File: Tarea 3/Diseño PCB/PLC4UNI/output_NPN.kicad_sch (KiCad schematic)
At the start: 3 parts

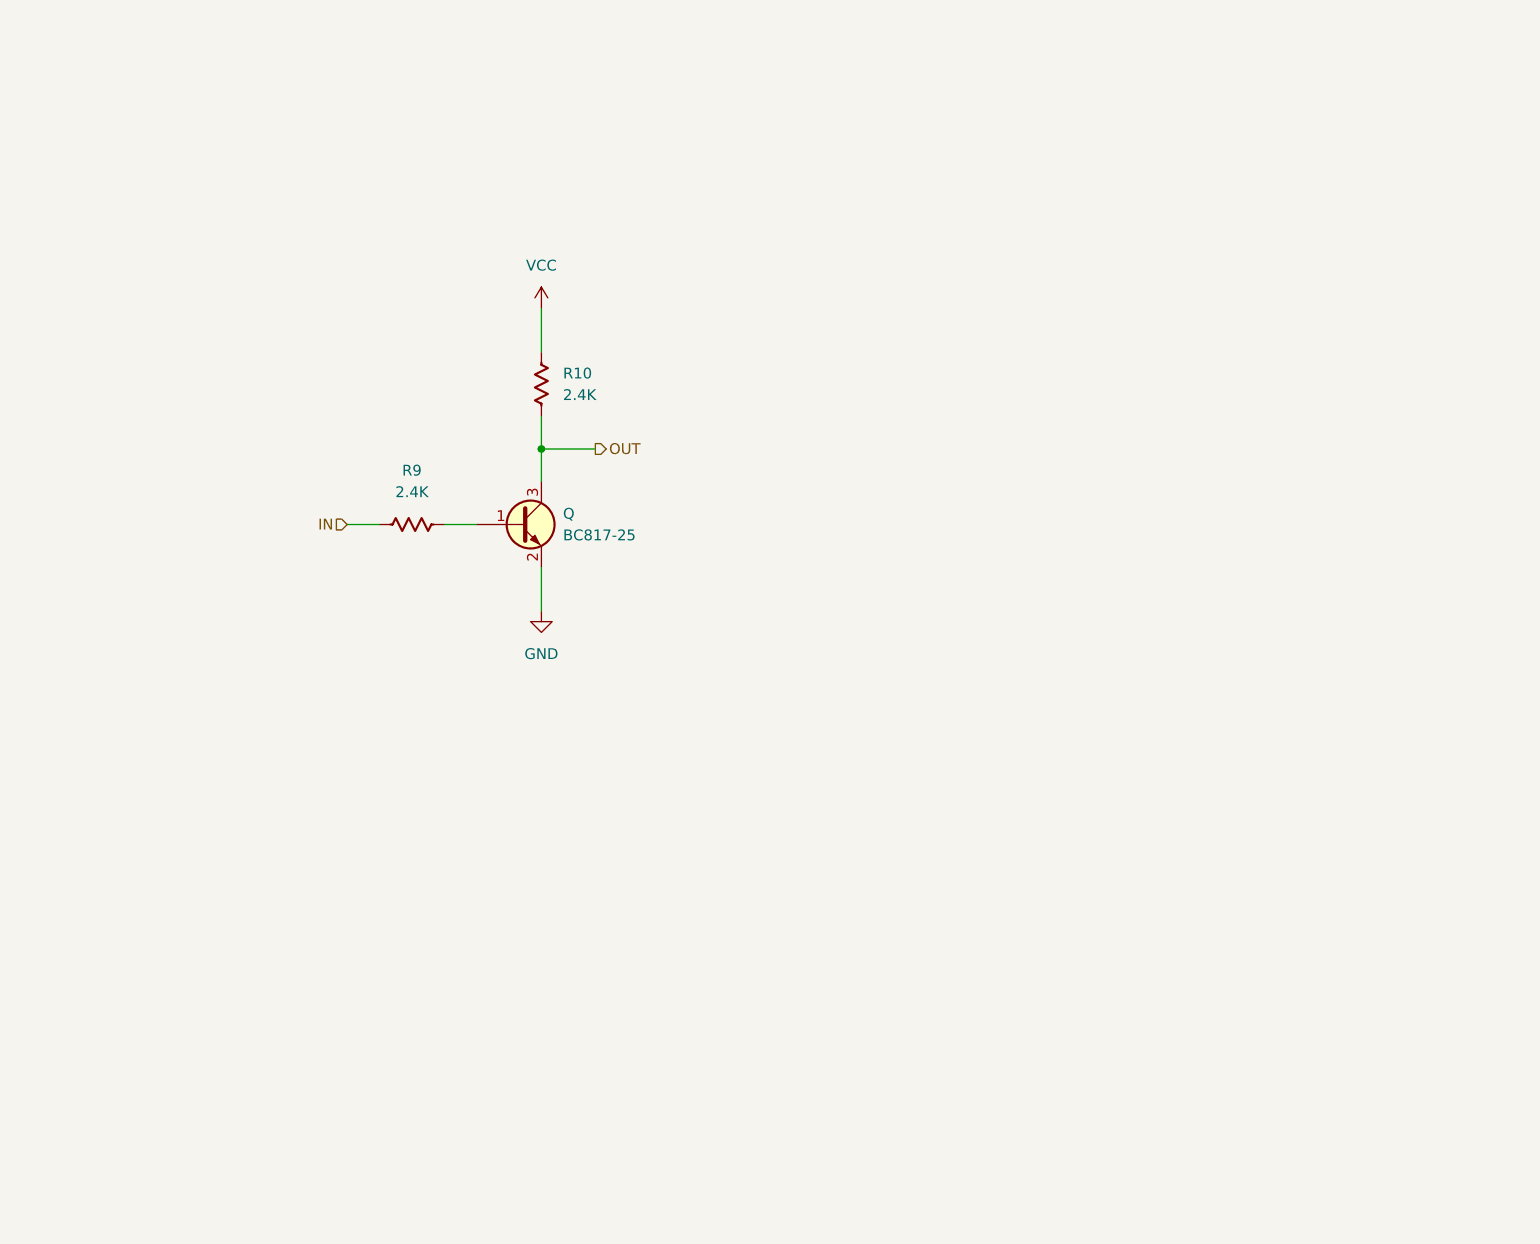
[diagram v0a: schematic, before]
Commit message: Tarea 3
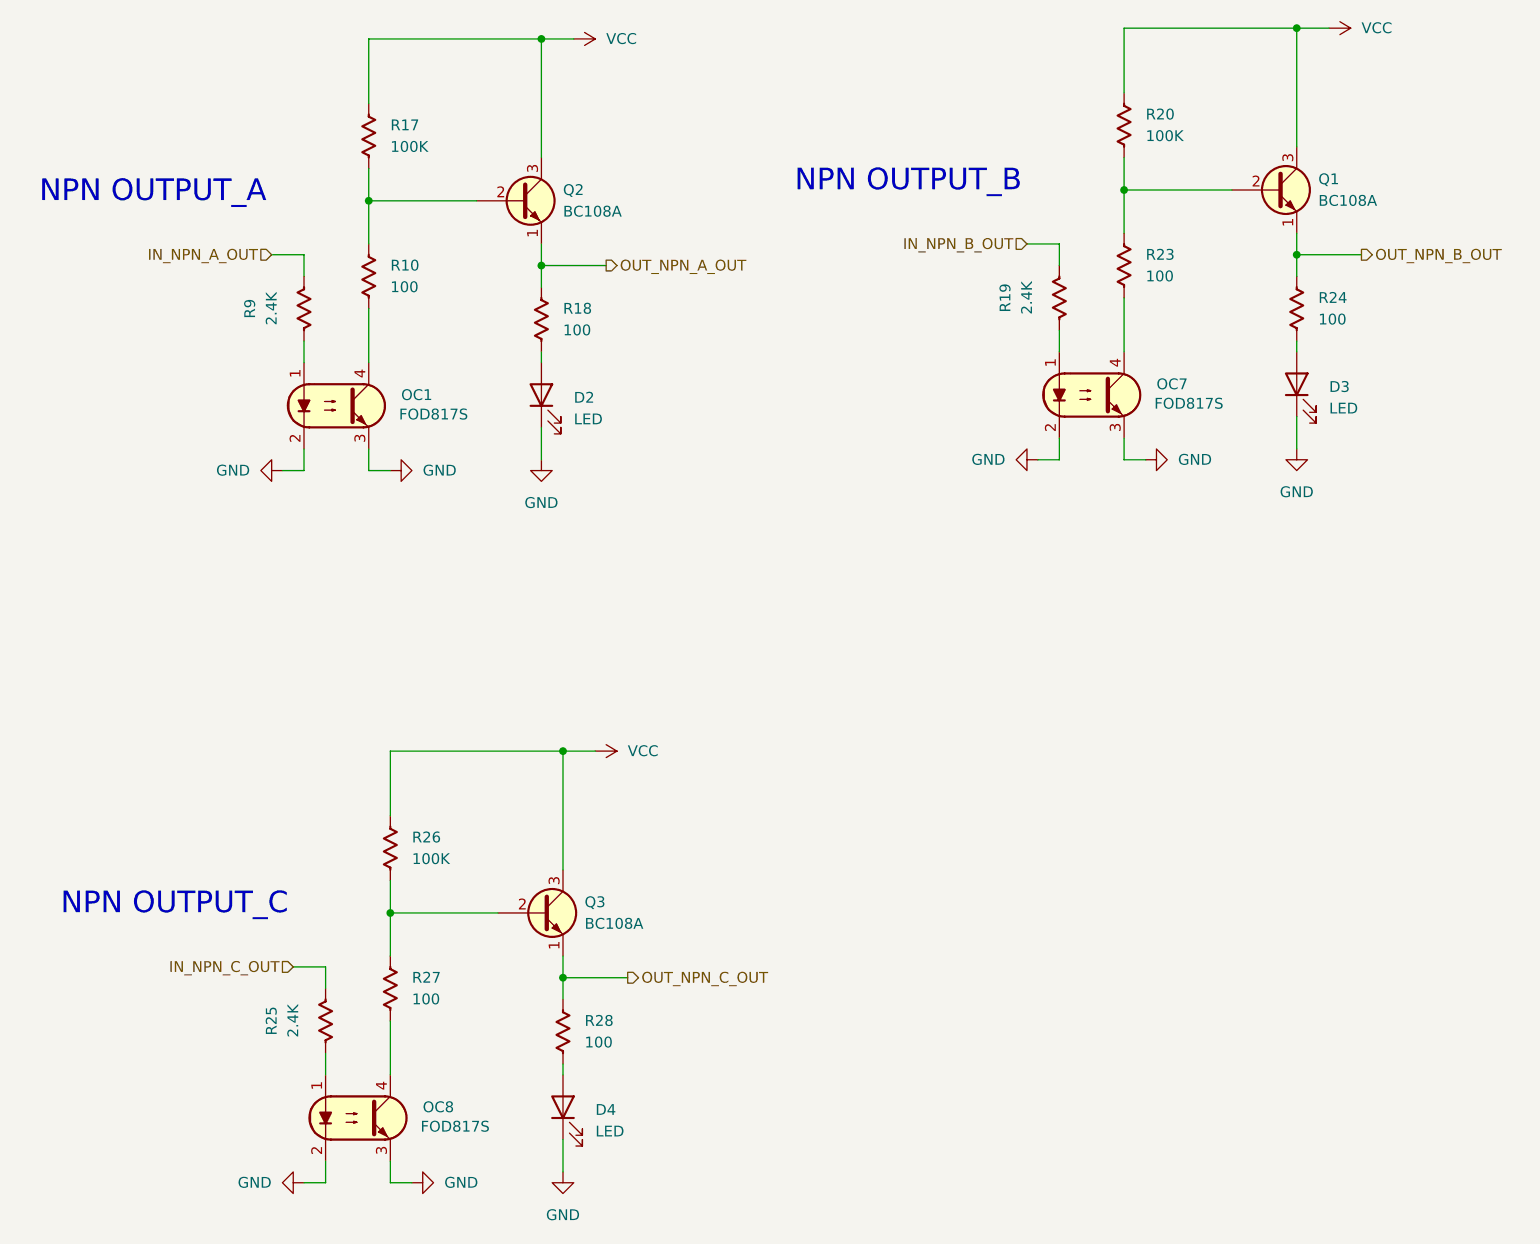
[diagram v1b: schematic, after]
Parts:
- removed Q: BC817-25, PCM_Package_TO_SOT_SMD_AKL:SOT-23, symbol PCM_Transistor_BJT_AKL:BC817-25
- added D2, D3, D4: LED, symbol Device:LED
- added OC1, OC7, OC8: FOD817S, PCM_Package_DIP_AKL:SMDIP-4_W9.53mm, symbol PCM_Optocoupler_AKL:FOD817S
- added Q1, Q2, Q3: BC108A, PCM_Package_TO_SOT_THT_AKL:TO-18-3_EBC, symbol PCM_Transistor_BJT_AKL:BC108A
- added R17, R20, R26: 100K, PCM_Resistor_SMD_AKL:R_0603_1608Metric, symbol PCM_Resistor_US_AKL:R_0603
- added R18, R23, R24, R27, R28: 100, PCM_Resistor_SMD_AKL:R_0603_1608Metric, symbol PCM_Resistor_US_AKL:R_0603
- added R19, R25: 2.4K, PCM_Resistor_SMD_AKL:R_0603_1608Metric, symbol PCM_Resistor_US_AKL:R_0603
- R10: value 2.4K -> 100
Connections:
- net GND: now also D2.1 (K), D3.1 (K), D4.1 (K), OC1.2, OC1.3, OC7.2, OC7.3, OC8.2, OC8.3
- net VCC: now also Q1.3 (C), Q2.3 (C), Q3.3 (C), R17.2, R20.2, R26.2; no longer R10.2
- net at R9.2: now also OC1.1
- net IN renamed IN_NPN_A_OUT
- net OUT: no longer names the net of R10.1
- net OUT: now also OC1.4
- new net: D4.2 (A), R28.1
- new net: Q1.2 (B), R20.1, R23.2
- new net: D3.2 (A), R24.1
- new net: D2.2 (A), R18.1
- new net: Q2.2 (B), R10.2, R17.1
- new net: OC7.1, R19.2
- new net: OC8.1, R25.2
- new net: OC7.4, R23.1
- new net: OC8.4, R27.1
- new net: Q3.2 (B), R26.1, R27.2
- new net IN_NPN_B_OUT: R19.1
- new net IN_NPN_C_OUT: R25.1
- new net OUT_NPN_A_OUT: Q2.1 (E), R18.2
- new net OUT_NPN_B_OUT: Q1.1 (E), R24.2
- new net OUT_NPN_C_OUT: Q3.1 (E), R28.2
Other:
- note added: "NPN OUTPUT_A"
- note added: "NPN OUTPUT_B"
- note added: "NPN OUTPUT_C"
- moved on the sheet: R10, R9
